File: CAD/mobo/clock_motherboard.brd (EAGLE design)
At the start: 68.6 x 53.3 mm, 32 parts, among them IC1 LM1086CT-5.0, IC2 LM1086CT-3.3, J2 2.1MMJACK, U1 ATMEGA328P_PDIP, U2 DS1307, Y2 32.768

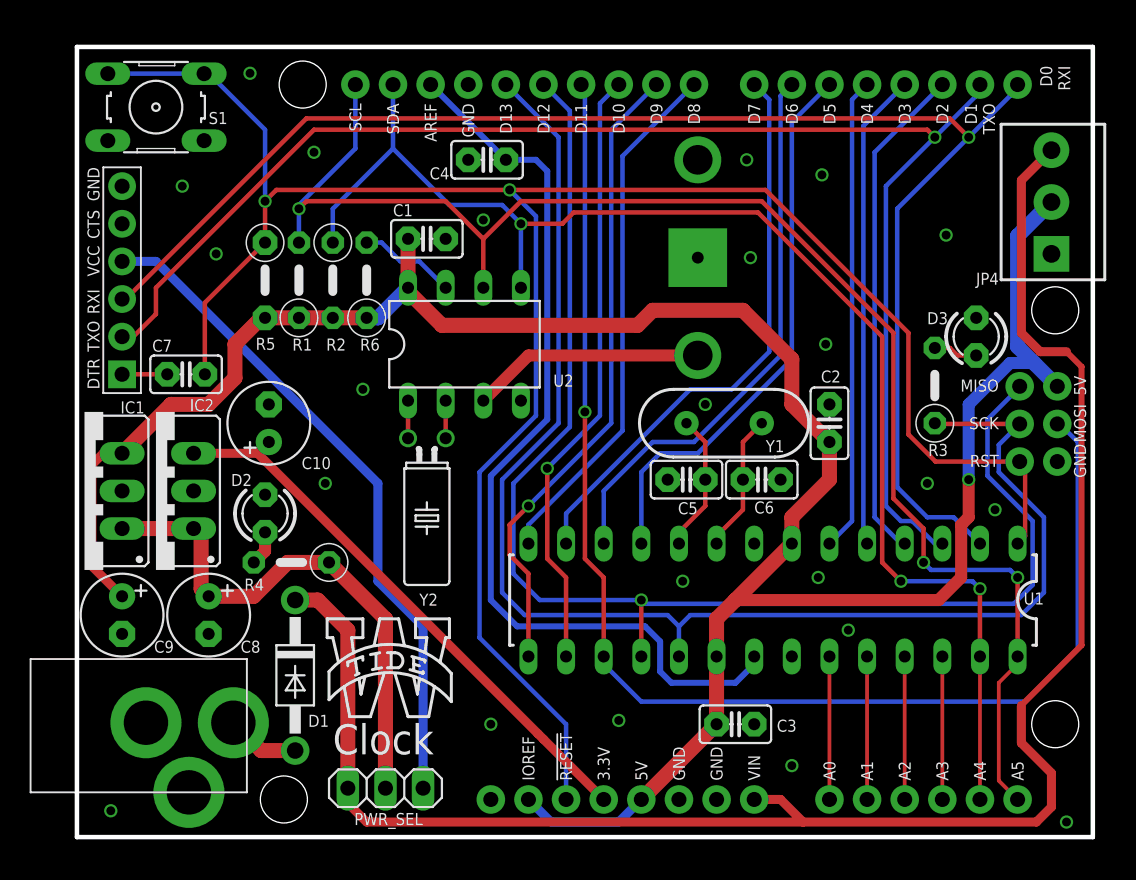
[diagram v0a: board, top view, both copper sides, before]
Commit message: Updating motherboard CAD files (OSHpark version)
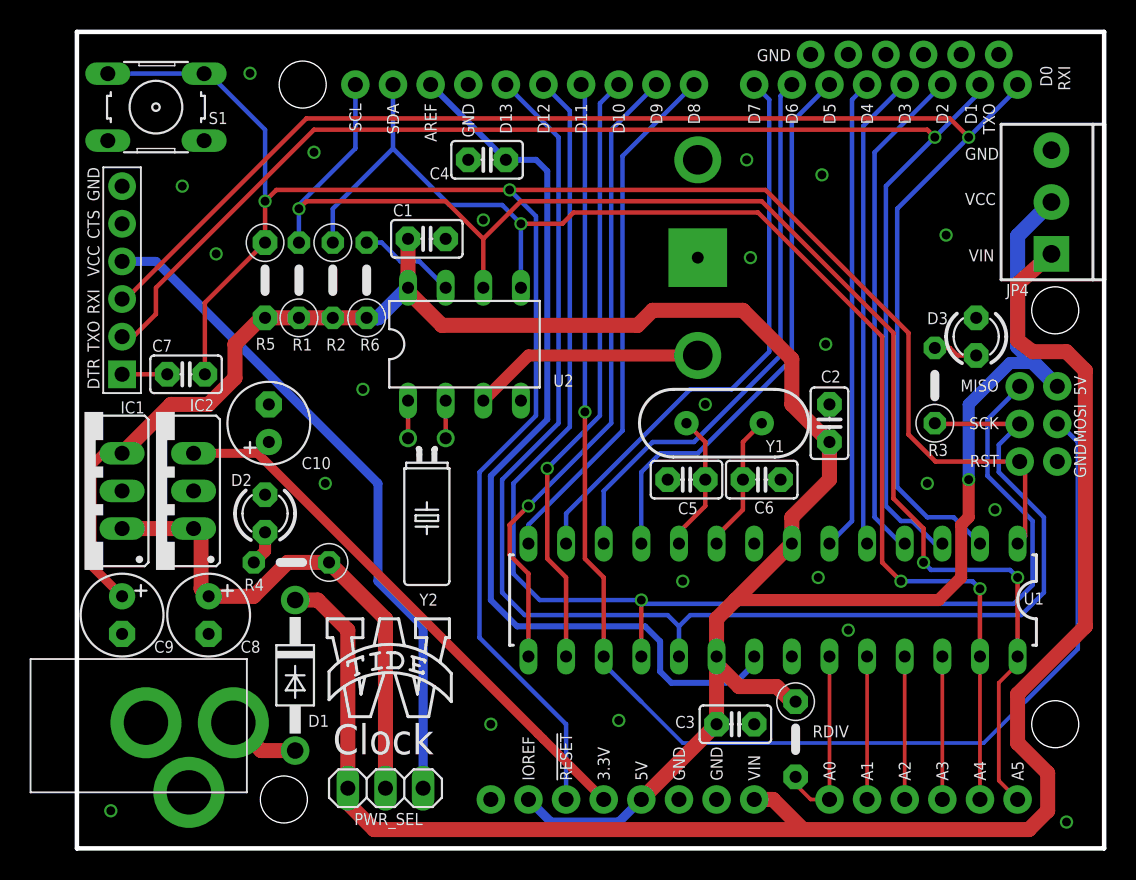
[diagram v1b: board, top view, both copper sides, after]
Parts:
- added GND: (no value), SparkFun-Connectors:1X06_NO_SILK
- added RDIV: 10K, rcl-ez:0207/5V
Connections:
- net A0: now also RDIV.2
- net GND: now also GND.1, GND.2, GND.3, GND.4, GND.5, GND.6, JP4.3; no longer JP4.1
- net VCC: now also RDIV.1
- net VIN: now also JP4.1; no longer JP4.3
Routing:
- net VCC: track 162.3 -> 168.7 mm
- net VIN: track 118.9 -> 113.4 mm
- net A0: track 9.65 -> 12.9 mm
- net D11/MOSI: track 90.1 -> 92.5 mm
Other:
- board size 68.6 x 53.3 mm -> 69.3 x 55.1 mm
- board text added: "GND"
- board text added: "VCC"
- board text added: "VIN"
